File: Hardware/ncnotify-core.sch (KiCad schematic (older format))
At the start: 42 parts, among them J1 5-1634503-1, J2 TC2030-CTX, J3 USB4110-GF-A, Q1 NX3008NBKS, SW1 SW_Push, SW2 SW_Push, U1 STM32L422CBT6, U2 TLV71333PDBV, U3 USBLC6-2SC6, U4 USBLC6-2SC6, X1 SMTU1632-LF, Y1 Q13FC1350000400

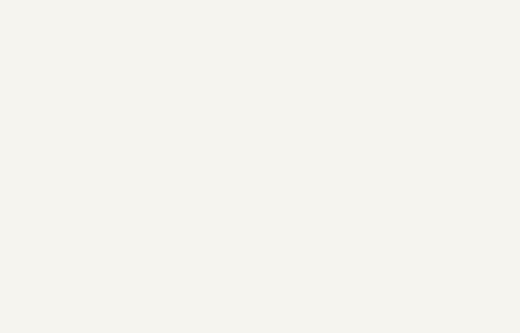
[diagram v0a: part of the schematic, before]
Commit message: bump to developing version v1.1
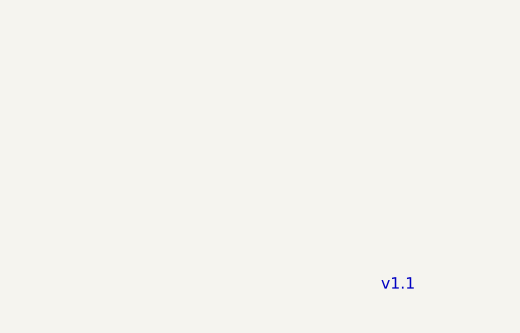
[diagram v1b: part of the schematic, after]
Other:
- note added: "v1.1"
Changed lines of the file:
@@
 	2150 1250 2050 1250
 Connection ~ 2050 1250
+Text Notes 10700 7650 0    50   ~ 0
+v1.1
 $EndSCHEMATC
